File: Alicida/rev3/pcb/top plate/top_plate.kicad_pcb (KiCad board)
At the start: 2 copper layers, 371.8 x 114.7 mm, 129 parts

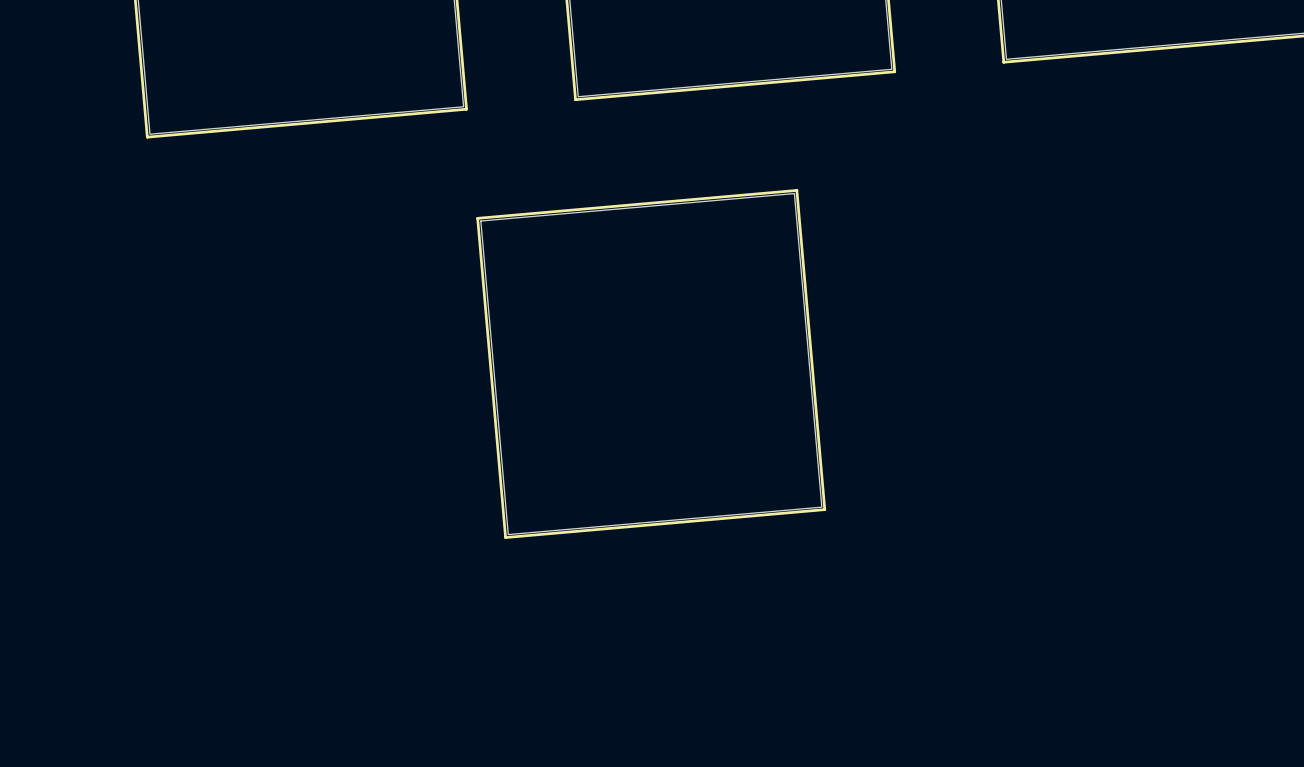
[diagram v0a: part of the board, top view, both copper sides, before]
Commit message: 3d update
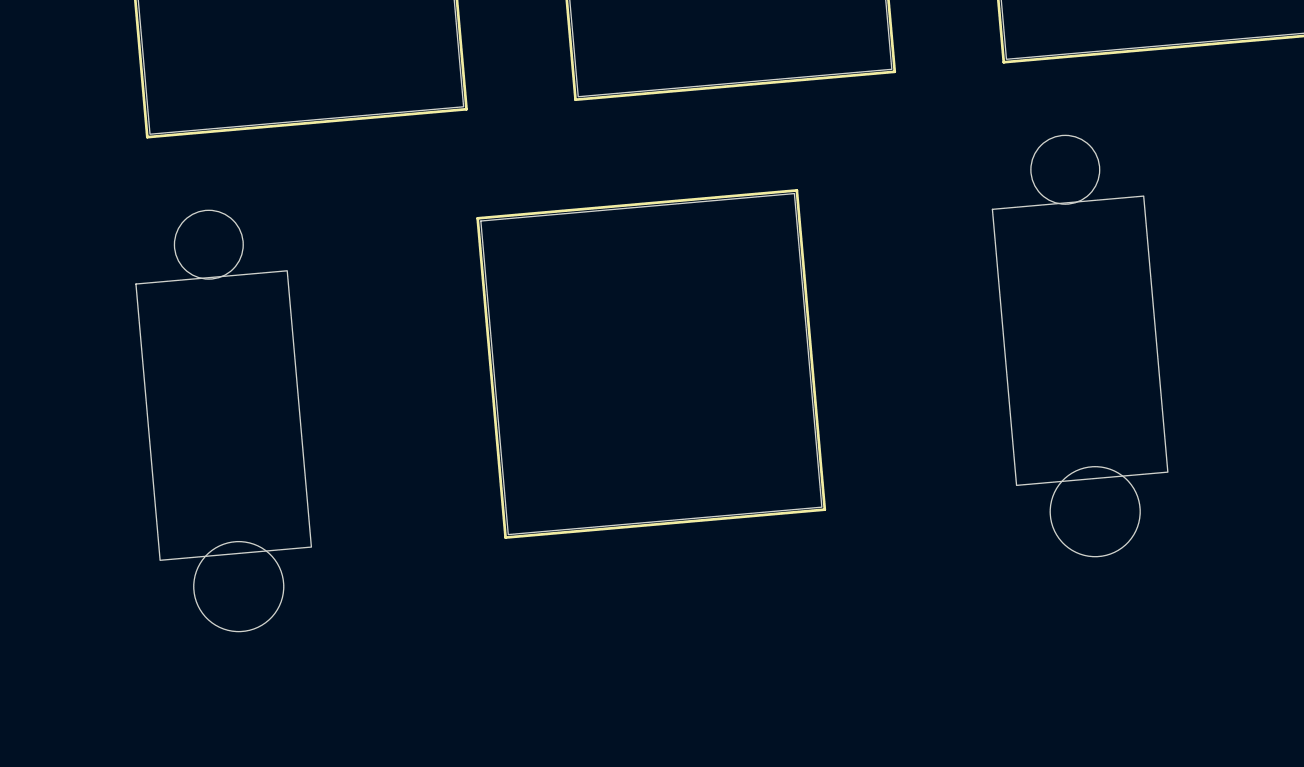
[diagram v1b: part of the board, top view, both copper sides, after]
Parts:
- added REF**: 3u top plate stab, Mounting_Keyboard_Stabilizer:3u top plate stab, F.Cu at (224.6, 179.5)
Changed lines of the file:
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@@
       (outputformat 1)
       (mirror false)
-      (drillshape 1)
+      (drillshape 0)
       (scaleselection 1)
-      (outputdirectory "")
+      (outputdirectory "gerber/")
     )
   )
@@
     )
   )
-  (footprint "keyboard_parts:nothing" (layer "F.Cu")
+  (footprint "Mounting_Keyboard_Stabilizer:3u top plate stab" (layer "F.Cu")
+    (at 224.64486 179.477934 5)
+    (attr smd)
+    (fp_text reference "REF**" (at 0.015 -0.5 5 unlocked) (layer "F.SilkS") hide
+        (effects (font (size 1 1) (thickness 0.1)))
+    )
+    (fp_text value "3u top plate stab" (at 0.015 1 5 unlocked) (layer "F.Fab") hide
+        (effects (font (size 1 1) (thickness 0.15)))
+    )
+    (fp_line (start -2.02 0.01) (end 1.98 0.01)
+      (stroke (width 0.1) (type solid)) (layer "Dwgs.User"))
+    (fp_line (start -0.02 2.01) (end -0.02 -1.99)
+      (stroke (width 0.1) (type solid)) (layer "Dwgs.User"))
+    (fp_line (start -22.445 -5.52) (end -22.445 6.78)
+      (stroke (width 0.1) (type solid)) (layer "Eco1.User"))
+    (fp_line (start -22.445 6.78) (end -15.695 6.78)
+      (stroke (width 0.1) (type solid)) (layer "Eco1.User"))
+    (fp_line (start -15.695 -5.52) (end -22.445 -5.52)
+      (stroke (width 0.1) (type solid)) (layer "Eco1.User"))
+    (fp_line (start -15.695 6.78) (end -15.695 -5.52)
+      (stroke (width 0.1) (type solid)) (layer "Eco1.User"))
+    (fp_line (start 15.655 -5.52) (end 15.655 6.78)
+      (stroke (width 0.1) (type solid)) (layer "Eco1.User"))
+    (fp_line (start 15.655 6.78) (end 22.405 6.78)
+      (stroke (width 0.1) (type solid)) (layer "Eco1.User"))
+    (fp_line (start 22.405 -5.52) (end 15.655 -5.52)
+      (stroke (width 0.1) (type solid)) (layer "Eco1.User"))
+    (fp_line (start 22.405 6.78) (end 22.405 -5.52)
+      (stroke (width 0.1) (type solid)) (layer "Eco1.User"))
+    (fp_rect (start -22.44 -5.52) (end -15.71 6.77)
+      (stroke (width 0.05) (type default)) (fill none) (layer "Edge.Cuts"))
+    (fp_rect (start 15.66 -5.51) (end 22.39 6.77)
+      (stroke (width 0.05) (type default)) (fill none) (layer "Edge.Cuts"))
+    (pad "" np_thru_hole circle (at -19.07 -6.975 5) (size 3.048 3.048) (drill 3.048) (layers "F&B.Cu" "*.Mask"))
+    (pad "" np_thru_hole circle (at -19.07 8.235 5) (size 3.9878 3.9878) (drill 3.9878) (layers "F&B.Cu" "*.Mask"))
+    (pad "" np_thru_hole circle (at 19.03 -6.975 5) (size 3.048 3.048) (drill 3.048) (layers "F&B.Cu" "*.Mask"))
+    (pad "" np_thru_hole circle (at 19.03 8.235 5) (size 3.9878 3.9878) (drill 3.9878) (layers "F&B.Cu" "*.Mask"))
+  )
+  (footprint "keyboard_parts:nothing" (layer "F.Cu")
